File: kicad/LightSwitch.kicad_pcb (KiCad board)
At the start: 2 copper layers, 42 x 70 mm, 26 parts, among them J2 RJ45, J3 RJ45, SW1 Pushbutton_LED, SW2 Pushbutton_LED, SW3 Pushbutton_LED, SW4 Pushbutton_LED, SW5 Pushbutton_LED, SW6 Pushbutton_LED, U1 LM1117-5.0, U2 ATtiny406-M, U3 SN65HVD232

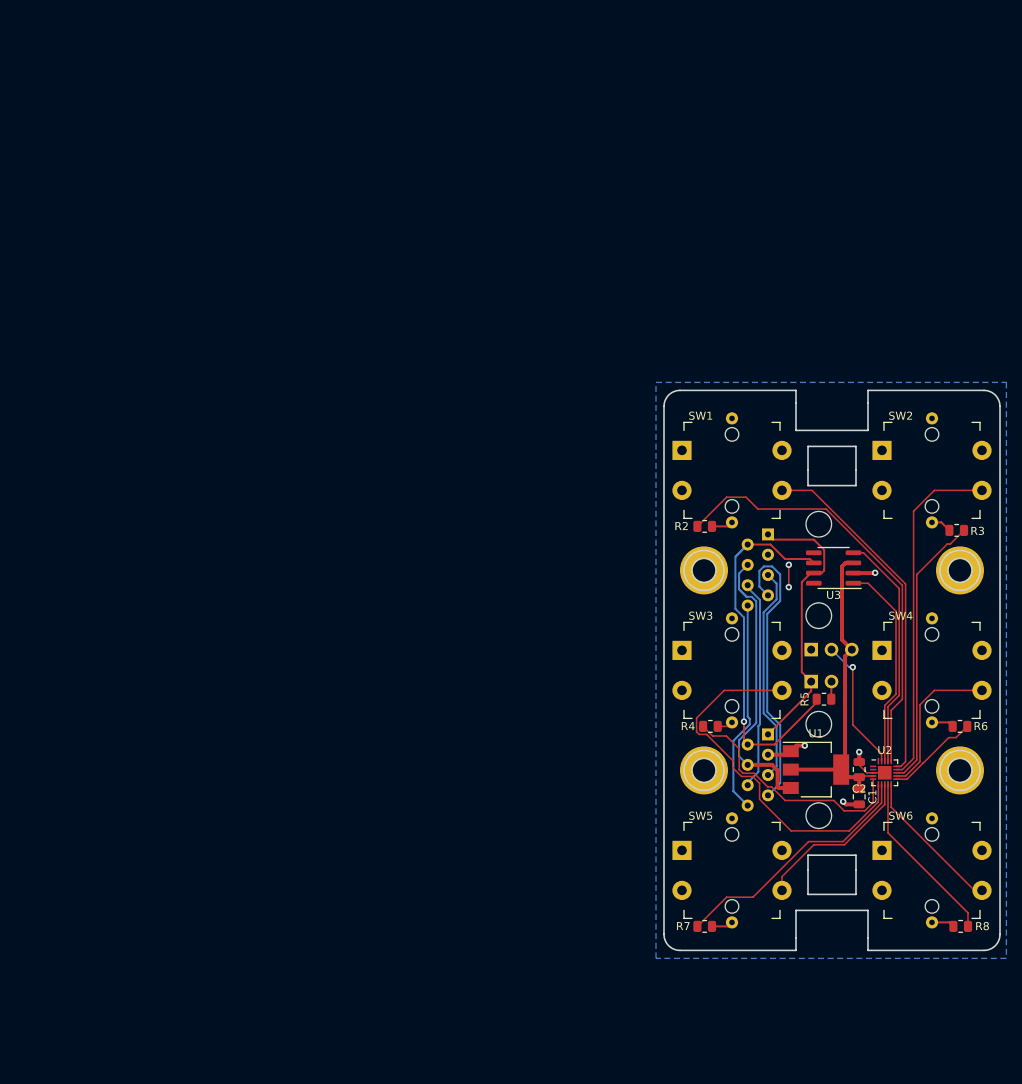
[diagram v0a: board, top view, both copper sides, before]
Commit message: Parking stuff, so I can contemplate the use of a nrf52840 _with_ DALI
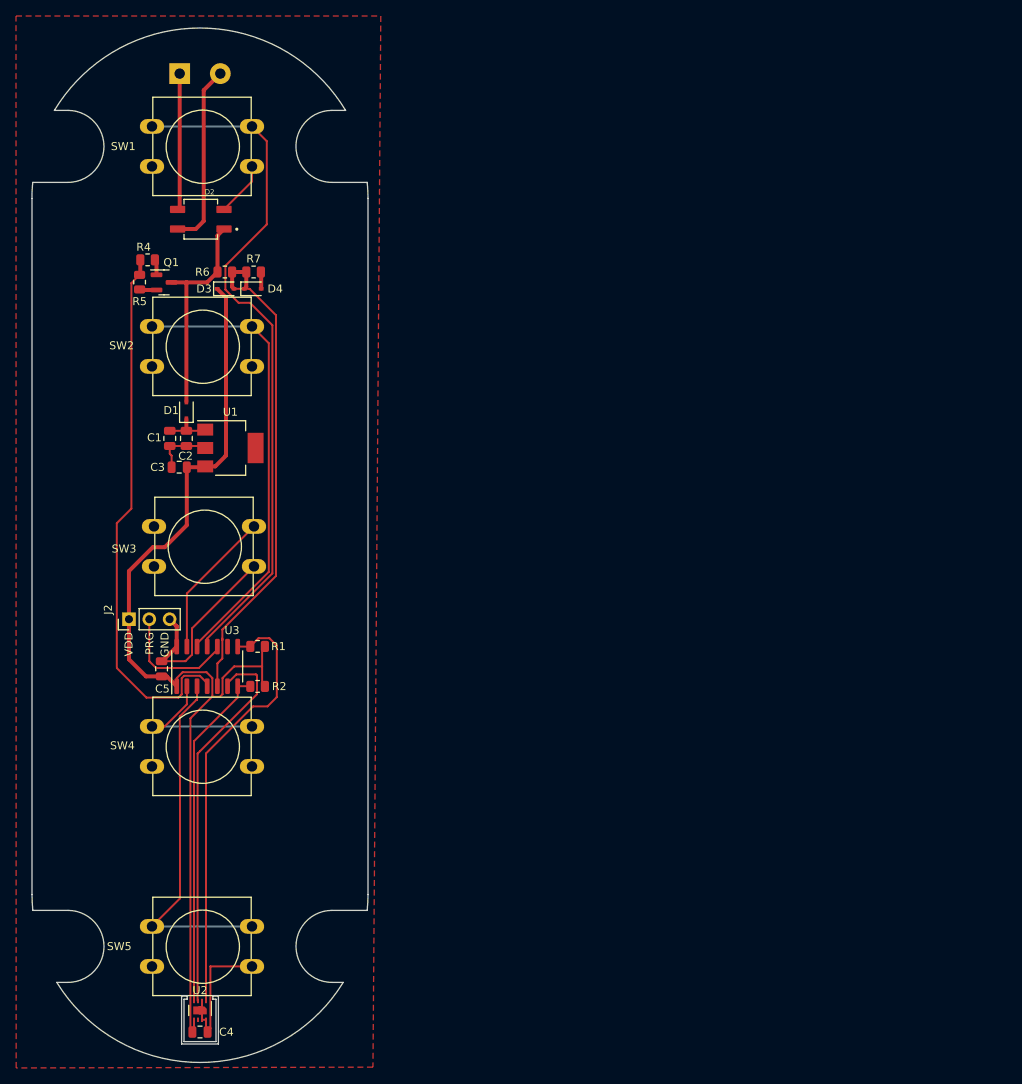
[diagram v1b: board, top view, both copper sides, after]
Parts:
- removed J3: RJ45, Connector_RJ:RJ45_Amphenol_54602-x08_Horizontal
- removed PROG: Conn_01x03_Male, Connector_PinHeader_2.54mm:PinHeader_1x03_P2.54mm_Vertical
- removed R3, R8: 220, Resistor_SMD:R_0805_2012Metric
- removed REF** (x4): MountingHole_3mm_Pad, MountingHole:MountingHole_3mm_Pad
- removed SW6: Pushbutton_LED, LightSwitch:12x12x7.3 LED Pushbutton
- removed TERM: Jumper, Connector_PinHeader_2.54mm:PinHeader_1x02_P2.54mm_Vertical
- added C3: 10u, Capacitor_SMD:C_0805_2012Metric, F.Cu at (118.4, 74.6)
- added C4: 0.1u, Capacitor_SMD:C_0805_2012Metric, F.Cu at (121.0, 145.2)
- added C5: 0.1u, Capacitor_SMD:C_0805_2012Metric, F.Cu at (116.2, 99.8)
- added D1: 1N4148WS, Diode_SMD:D_SOD-323, F.Cu at (119.3, 67.5)
- added D2: D_Bridge_+-AA, imported_modules:SOIC245P670X290-4N, F.Cu at (121.1, 43.6)
- added D3: 1N4148WS, Diode_SMD:D_SOD-323, F.Cu at (124.2, 52.3)
- added D4: 1N4148WS, Diode_SMD:D_SOD-323, F.Cu at (127.6, 52.3)
- added J1: Screw_Terminal_01x02, TerminalBlock_Phoenix:TerminalBlock_Phoenix_MKDS-1,5-2-5.08_1x02_P5.08mm_Horizontal, B.Cu at (118.5, 25.4)
- added Q1: MMBT2222A, Package_TO_SOT_SMD:SOT-23, F.Cu at (116.5, 51.5)
- added R1: 4.7K, Resistor_SMD:R_0805_2012Metric, F.Cu at (128.2, 97.0)
- C1: value 0.1u -> 10u
- C2: value 10u -> 0.1u
- J2: value RJ45 -> Conn_01x03_Male; footprint Connector_RJ:RJ45_Amphenol_54602-x08_Horizontal -> Connector_PinHeader_2.54mm:PinHeader_1x03_P2.54mm_Vertical; moved to F.Cu
- R2: value 220 -> 4.7K
- R4: value 220 -> 120
- R5: value 120 -> 1K
- R6: value 220 -> 27K
- R7: value 220 -> 2K
- SW1, SW2, SW3, SW4, SW5: value Pushbutton_LED -> SW_Push; footprint LightSwitch:12x12x7.3 LED Pushbutton -> Button_Switch_THT:SW_PUSH-12mm
- U1: value LM1117-5.0 -> LM2936-3.3; footprint Package_TO_SOT_SMD:SOT-223-3_TabPin2 -> Package_TO_SOT_SMD:SOT-223
- U2: value ATtiny406-M -> SHT35-DIS; footprint Package_DFN_QFN:VQFN-20-1EP_3x3mm_P0.4mm_EP1.7x1.7mm -> Sensor_Humidity:Sensirion_DFN-8-1EP_2.5x2.5mm_P0.5mm_EP1.1x1.7mm
- U3: value SN65HVD232 -> ATtiny804-SS; footprint Package_SO:SOIC-8_3.9x4.9mm_P1.27mm -> Package_SO:SOIC-14_3.9x8.7mm_P1.27mm
- moved R6 108.0 mm to (124.1, 50.2), turned to 0 degrees
- moved R5 100.2 mm to (113.5, 51.5), turned to -90 degrees
- moved R7 99.4 mm to (127.7, 50.2)
- moved SW2 99.1 mm to (115.0, 57.0)
- moved SW4 97.8 mm to (115.0, 107.0)
- moved C1 97.1 mm to (117.2, 71.0)
- moved C2 93.7 mm to (119.3, 71.0), turned to -90 degrees
- moved R4 91.4 mm to (114.5, 48.7), turned to 180 degrees
- moved U2 90.6 mm to (121.0, 142.5), turned to -90 degrees
- moved SW1 84.3 mm to (115.0, 32.0)
- moved U1 83.5 mm to (124.8, 72.2)
- moved J2 81.2 mm to (112.1, 93.6), turned to 90 degrees
- moved U3 79.3 mm to (121.9, 99.5), turned to 90 degrees
- moved SW3 74.5 mm to (115.2, 82.0)
- moved SW5 72.8 mm to (115.0, 132.0)
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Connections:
- C1 pad 1: VDD -> Net-(C1-Pad1)
- C2 pad 1: VDD -> Net-(C1-Pad1)
- J2 pad 1: /CANH -> VDD
- J2 pad 2: /CANL -> /PROG
- R2 pad 1: /LED1 -> VDD
- R2 pad 2: Net-(R2-Pad2) -> /SCL
- R4 pad 1: /LED3 -> Net-(Q1-Pad1)
- R4 pad 2: Net-(R4-Pad2) -> /DALI_TX
- R5 pad 1: Net-(JP1-Pad2) -> /DALI_TX
- R5 pad 2: /CANL -> GND
- R6 pad 1: /LED4 -> /DALI+
- R6 pad 2: Net-(R6-Pad2) -> /DALI_RX
- R7 pad 1: /LED5 -> /DALI_RX
- R7 pad 2: Net-(R7-Pad2) -> GND
- SW1 pad 1: GND -> /SW1
- SW1 pad 2: Net-(SW1-Pad2) -> GND
- SW2 pad 1: GND -> /SW2
- SW2 pad 2: Net-(SW2-Pad2) -> GND
- SW3 pad 1: GND -> /SW3
- SW3 pad 2: Net-(SW3-Pad2) -> GND
- SW4 pad 1: GND -> /SW4
- SW4 pad 2: Net-(SW4-Pad2) -> GND
- SW5 pad 1: GND -> /SW5
- SW5 pad 2: Net-(SW5-Pad2) -> GND
- U1 pad 1: GND -> Net-(C1-Pad1)
- U1 pad 2: VDD -> GND
- U1 pad 3: /VIN -> VDD
- U2 pad 1: Net-(U2-Pad1) -> /SDA
- U2 pad 2: Net-(U2-Pad2) -> GND
- U2 pad 3: GND -> /TEMP_ALERT
- U2 pad 4: VDD -> /SCL
- U2 pad 5: /LED3 -> VDD
- U2 pad 6: /SW3 -> unconnected-(U2-Pad6)
- U2 pad 7: /LED5 -> GND
- U2 pad 8: /SW5 -> GND
- U2 pad 9: /LED6 -> GND
- U3 pad 1: /CAN_TX -> VDD
- U3 pad 2: GND -> /SW4
- U3 pad 3: VDD -> /SW5
- U3 pad 4: /CAN_RX -> /DALI_TX
- U3 pad 5: Net-(U3-Pad5) -> /DALI_RX
- U3 pad 6: /CANL -> /TEMP_ALERT
- U3 pad 7: /CANH -> /SCL
- U3 pad 8: Net-(U3-Pad8) -> /SDA
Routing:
- net VDD: track 40.3 -> 129.6 mm
- net /DALI_TX: track 0.00 -> 68.0 mm
- net /DALI_RX: track 0.00 -> 62.4 mm
- net /SDA: track 0.00 -> 54.8 mm
- net /LED1: track 54.3 -> 0.00 mm
- net /CANL: track 50.8 -> 0.00 mm, vias 1 -> 0
- net /TEMP_ALERT: track 0.00 -> 48.3 mm
- net /SW1: track 43.9 -> 87.5 mm
- net GND: track 18.0 -> 61.2 mm, vias 6 -> 0
- net /SCL: track 0.00 -> 43.1 mm
- net /VIN: track 37.0 -> 0.00 mm
- net Net-(J2-Pad7): track 36.3 -> 0.00 mm
- net /CANH: track 35.6 -> 0.00 mm
- net /LED2: track 34.6 -> 0.00 mm
- net /LED5: track 31.7 -> 0.00 mm
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- added copper zone on F.Cu, net GND
- removed copper zone on B.Cu, net GND
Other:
- board size 42 x 70 mm -> 42 x 129.3 mm
- net class Default removed
- board text added: "GND"
- board text added: "PRG"
- board text added: "VDD"
